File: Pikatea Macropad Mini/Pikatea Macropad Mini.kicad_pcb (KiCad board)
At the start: 2 copper layers, 125.1 x 25 mm, 40 parts, among them J1 AVR-ISP-6, J2 Conn_01x02_Male, J3 Conn_01x02_Male, J4 Conn_01x03_Male, J5 Conn_01x03_Male, J6 Conn_01x04_Male, SW1 SW_DPST, SW2 Rotary_Encoder_Switch, SW3 SW_SPST, U1 ATMEGA32U4-EP, U2 AMS1117-3.3, U3 74LVC125APW,118, X1 16MHz

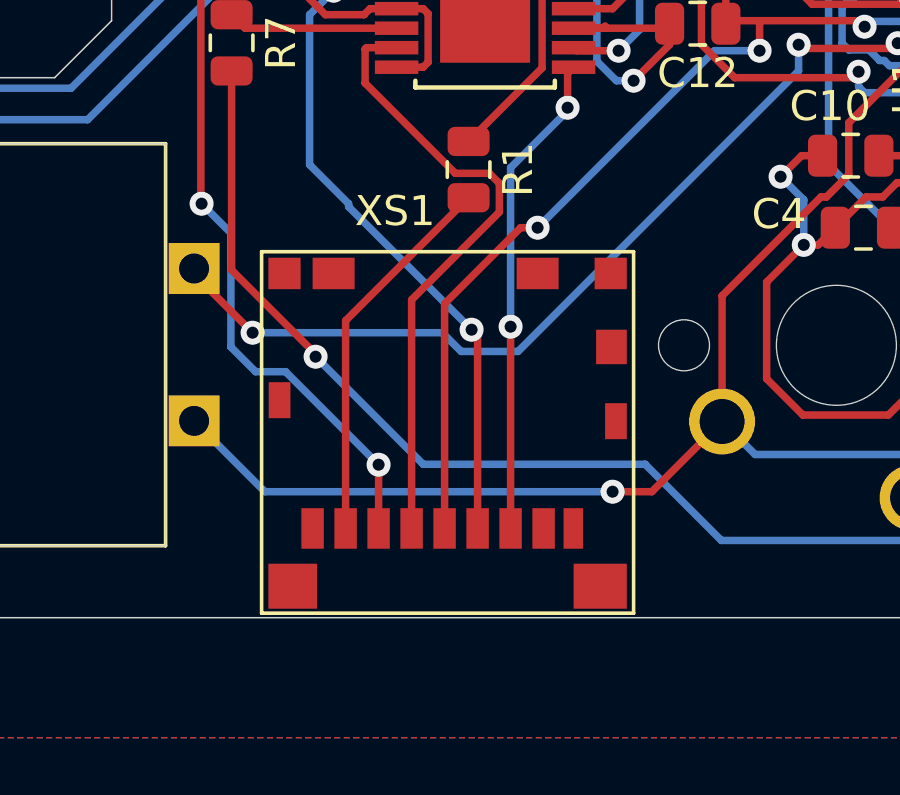
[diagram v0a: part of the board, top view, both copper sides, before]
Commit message: updates
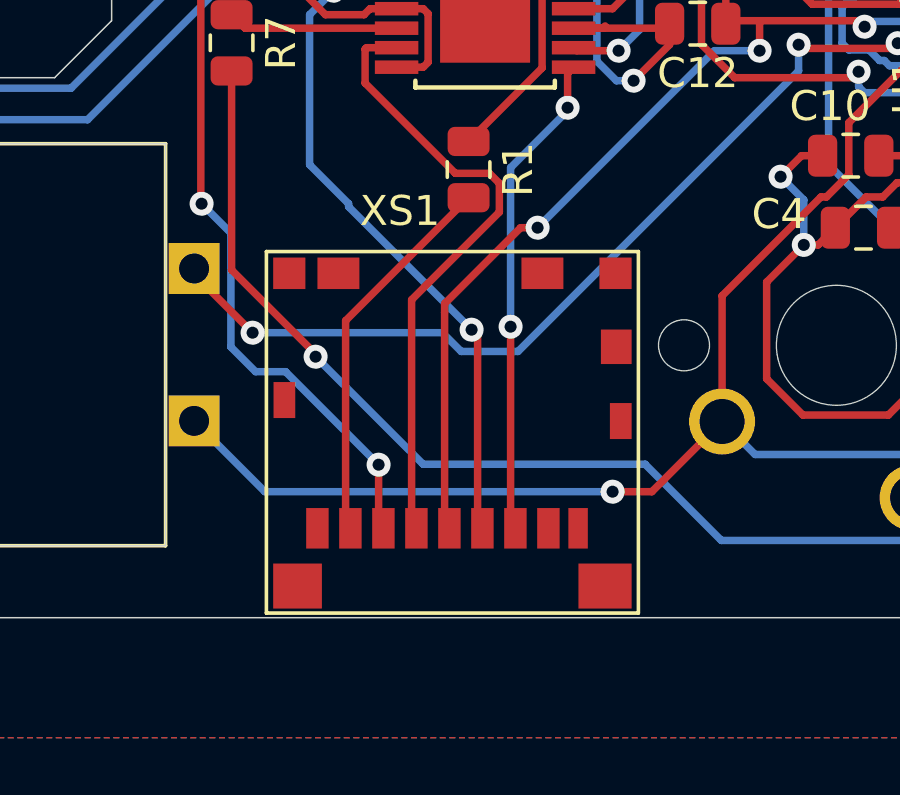
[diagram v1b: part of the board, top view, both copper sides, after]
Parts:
- moved XS1 0.16 mm to (118.1, 102.0)
